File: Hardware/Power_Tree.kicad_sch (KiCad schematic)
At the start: 22 parts, among them J1 BATTERY, J10 VCC, J2 USB_C_Receptacle_USB2.0_14P, J8 GND, J9 VDD, Q1 PMOS, Q2 PMOS, SW1 ON/OFF MECH, U1 AMS1117-3.3, U2 USBLC6-2

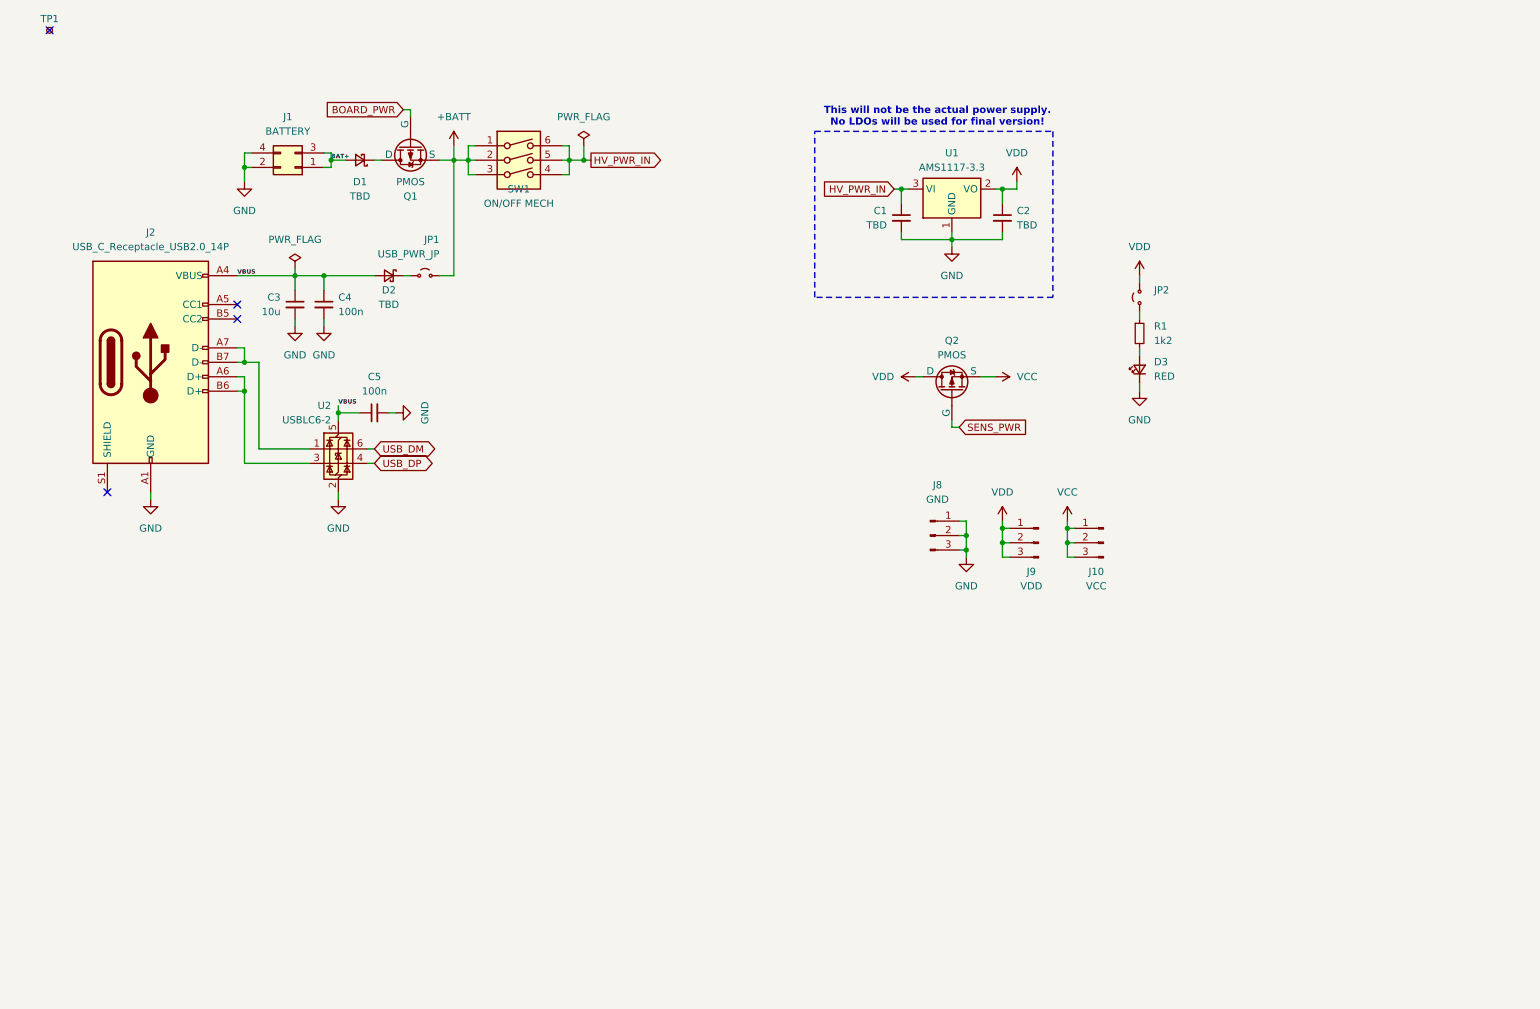
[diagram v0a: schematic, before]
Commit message: Working on power source
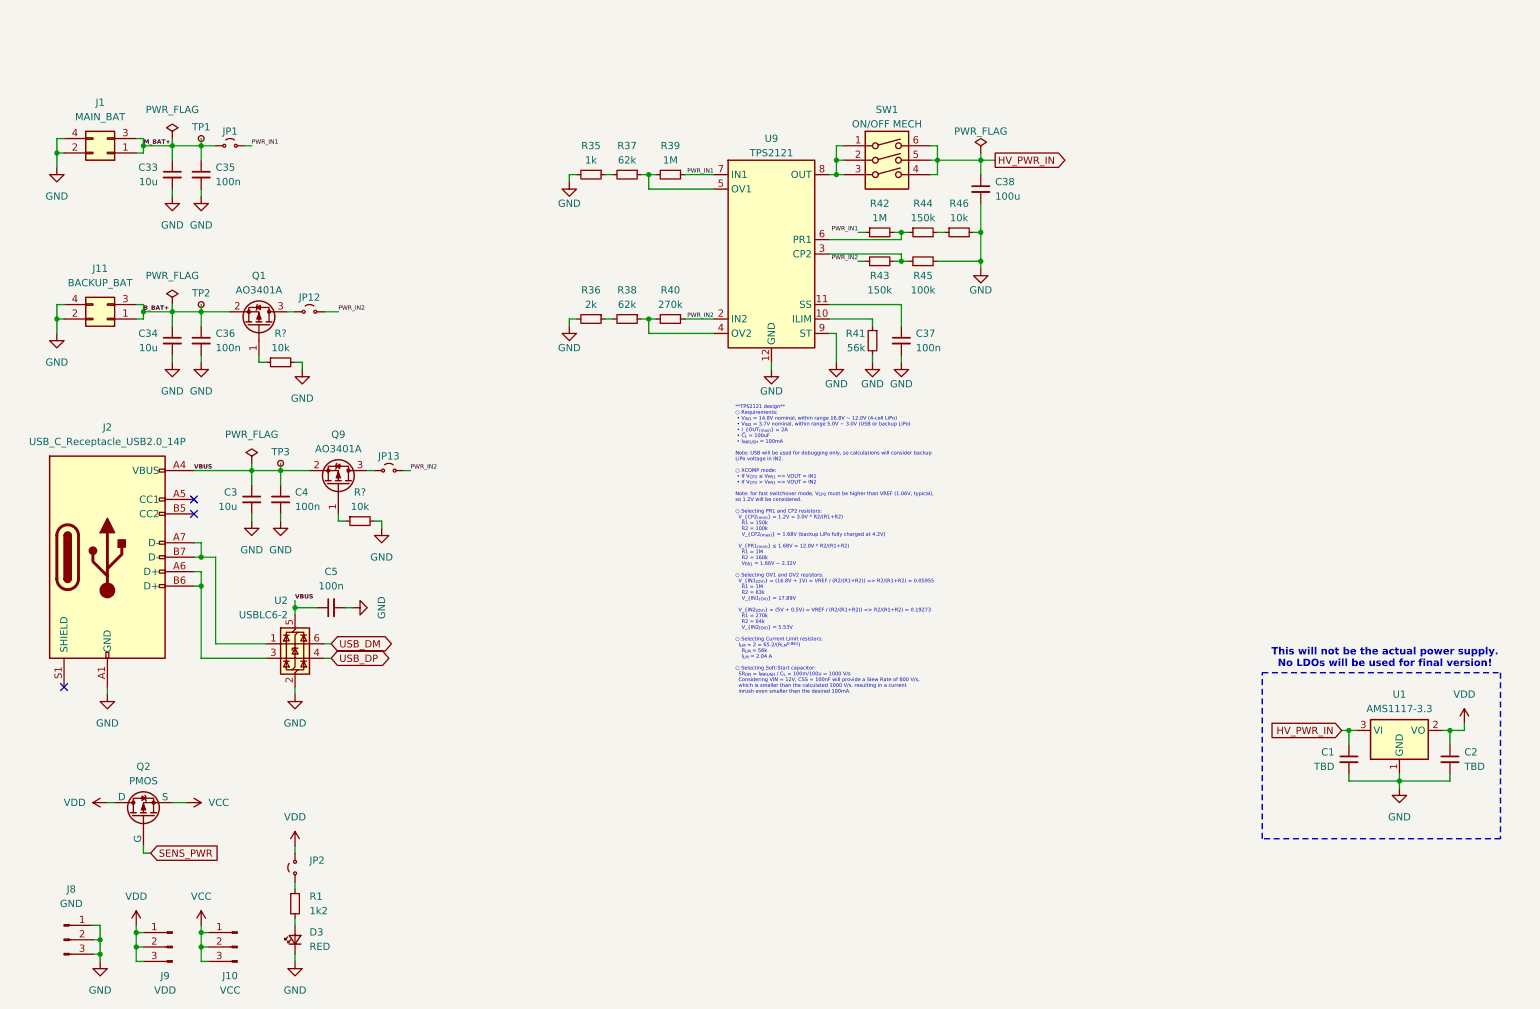
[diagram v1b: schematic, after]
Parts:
- removed D1, D2: TBD, Diode_SMD:D_SOD-123, symbol Device:D_Schottky_Small
- removed Q1: PMOS, Package_TO_SOT_SMD:SOT-23, symbol Simulation_SPICE:PMOS
- added C33, C34: 10u, Capacitor_SMD:C_0402_1005Metric, symbol Device:C_Small
- added C35, C36, C37: 100n, Capacitor_SMD:C_0402_1005Metric, symbol Device:C_Small
- added C38: 100u, Capacitor_SMD:C_0402_1005Metric, symbol Device:C_Small
- added J11: BACKUP_BAT, Connector_Molex:Molex_Micro-Fit_3.0_43045-0412_2x02_P3.00mm_Vertical, symbol Connector_Generic:Conn_02x02_Odd_Even
- added JP1, JP12: USB_PWR_JP, Jumper:SolderJumper-2_P1.3mm_Open_RoundedPad1.0x1.5mm, symbol Jumper:Jumper_2_Small_Open
- added Q1, Q9: AO3401A, Package_TO_SOT_SMD:SOT-23, symbol Transistor_FET:AO3401A
- added R35: 1k, Resistor_SMD:R_0402_1005Metric, symbol Device:R_Small
- added R36: 2k, Resistor_SMD:R_0402_1005Metric, symbol Device:R_Small
- added R37, R38: 62k, Resistor_SMD:R_0402_1005Metric, symbol Device:R_Small
- added R39, R42: 1M, Resistor_SMD:R_0402_1005Metric, symbol Device:R_Small
- added R40: 270k, Resistor_SMD:R_0402_1005Metric, symbol Device:R_Small
- added R41: 56k, Resistor_SMD:R_0402_1005Metric, symbol Device:R_Small
- added R43, R44: 150k, Resistor_SMD:R_0402_1005Metric, symbol Device:R_Small
- added R45: 100k, Resistor_SMD:R_0402_1005Metric, symbol Device:R_Small
- added R46, R? (x2): 10k, Resistor_SMD:R_0402_1005Metric, symbol Device:R_Small
- added TP2, TP3: TestPoint_Small, TestPoint:TestPoint_Pad_D1.5mm, symbol Connector:TestPoint_Small
- added U9: TPS2121, BRS_Footprints:VQFN-HR, symbol BRS_Library:TPS2121
- C1, C2, C3, C4, C5: footprint Capacitor_SMD:C_0603_1608Metric -> Capacitor_SMD:C_0402_1005Metric
- J1: value BATTERY -> MAIN_BAT
- JP2: footprint BRS_Footprints:SMD_SolderJumper_Small -> BRS_Footprints:SMD_SolderJumper_Micro
- R1: footprint Resistor_SMD:R_0603_1608Metric -> Resistor_SMD:R_0402_1005Metric
- renumbered JP1 to JP13
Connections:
- net BAT+ is gone; now on net M_BAT+: J1.1 (Pin_1), J1.3 (Pin_3)
- net GND: now also C33.2, C34.2, C35.2, C36.2, C37.2, C38.2, J11.2 (Pin_2), J11.4 (Pin_4), R35.2, R36.2, R41.2, R45.2, R46.2, R?.2, R?.2, U9.12 (GND), U9.9 (ST)
- net HV_PWR_IN: now also C38.1
- net VBUS: now also Q9.2 (S), TP3.1
- net M_BAT+: now reaches TP1.1
- net M_BAT+: now also C33.1, C35.1, JP1.1 (A)
- net at JP13.1 (A): now also Q9.3 (D)
- net +BATT: no longer names the net of SW1.1, SW1.2, SW1.3
- net +BATT: now also U9.1 (OUT), U9.8 (OUT); no longer JP13.2 (B)
- new net: R37.1, R39.2, U9.5 (OV1)
- new net: R35.1, R37.2
- new net: R43.2, R45.1, U9.3 (CP2)
- new net: R44.2, R46.1
- new net: R41.1, U9.10 (ILIM)
- new net: C37.1, U9.11 (SS)
- new net: R38.1, R40.2, U9.4 (OV2)
- new net: R42.2, R44.1, U9.6 (PR1)
- new net: Q1.1 (G), R?.1
- new net: JP12.1 (A), Q1.3 (D)
- new net: R36.1, R38.2
- new net: Q9.1 (G), R?.1
- new net B_BAT+: C34.1, C36.1, J11.1 (Pin_1), J11.3 (Pin_3), Q1.2 (S), TP2.1
- new net PWR_IN1: JP1.2 (B), R39.1, R42.1, U9.7 (IN1)
- new net PWR_IN2: JP12.2 (B), JP13.2 (B), R40.1, R43.1, U9.2 (IN2)
- no-connect marks 4 -> 3
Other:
- note added: "**TPS2121 design** ○ Requirements: • V_{IN1} = 14.8V nominal, within range 16.8V ~ 12.0V (4-cell LiPo) • V_{IN2} = 3.7V nominal, within range 5.0V ~ 3.0V (USB or backup LiPo) • I_{OUT_{(max)}} = 2A • C_{L} = 100uF • I_{INRUSH} = 100mA Note: USB will be used for debugging only, so calculations will consider backup LiPo voltage in IN2. ○ XCOMP mode: • If V_{CP2} ≤ V_{PR1} => VOUT = IN1 • If V_{CP2}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"
- moved on the sheet: C1, C2, C3, C4, C5, D3, J1, J10, J2, J8, J9, JP13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
